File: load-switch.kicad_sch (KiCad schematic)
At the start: 18 parts, among them IC3 TPS2H160AQPWPRQ1, IC4 TPS2H160AQPWPRQ1

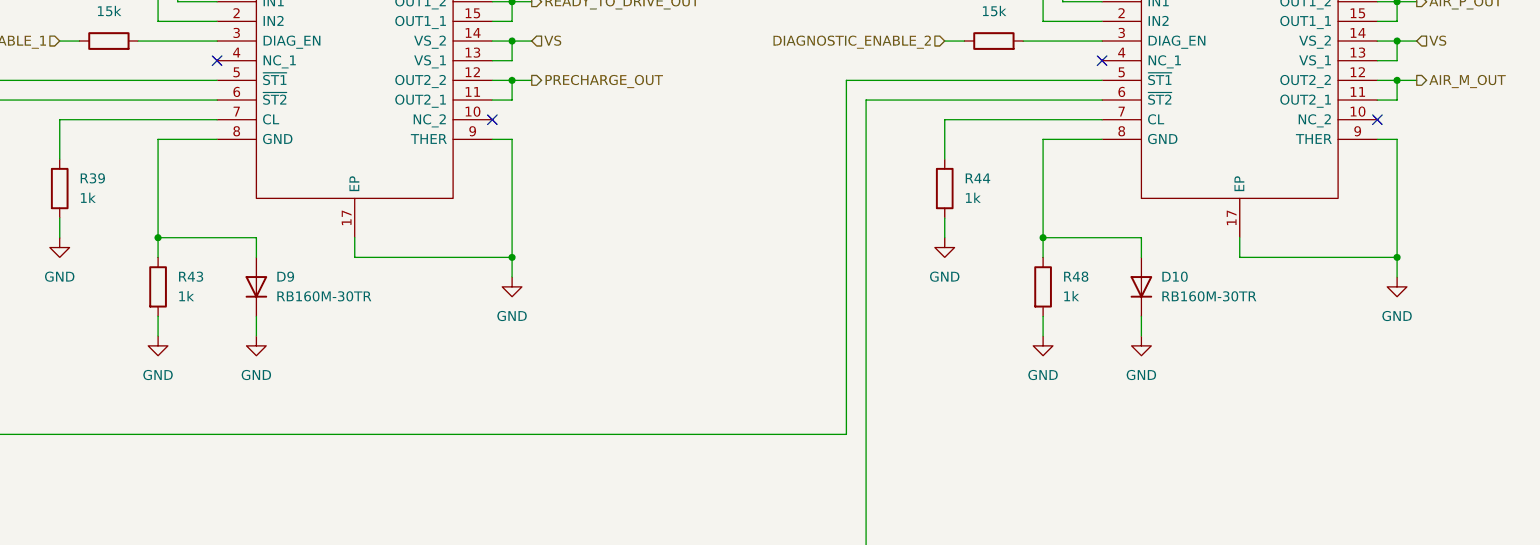
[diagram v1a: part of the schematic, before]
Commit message: サーマルパッドの接続先変更
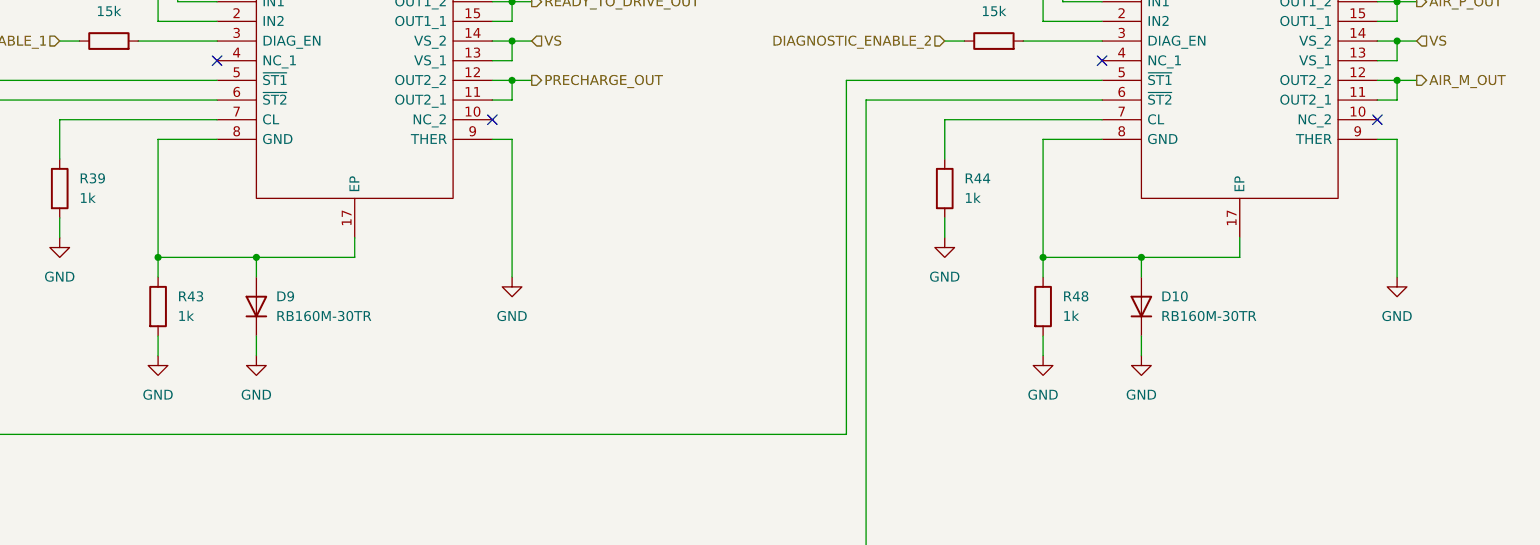
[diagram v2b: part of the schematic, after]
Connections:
- net GND: no longer IC3.17 (EP), IC4.17 (EP)
- net at D9.2 (A), IC3.8 (GND), R43.1: now also IC3.17 (EP)
- net at D10.2 (A), IC4.8 (GND), R48.1: now also IC4.17 (EP)
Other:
- moved on the sheet: D10, D9, R43, R48
